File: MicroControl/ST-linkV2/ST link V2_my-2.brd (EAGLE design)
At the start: 57.4 x 22.5 mm, 37 parts, among them IC1 LD117-3.3, Q1 8000 kHz, U1 STM32F103CBT6, X2 CON-PH12-EDGE

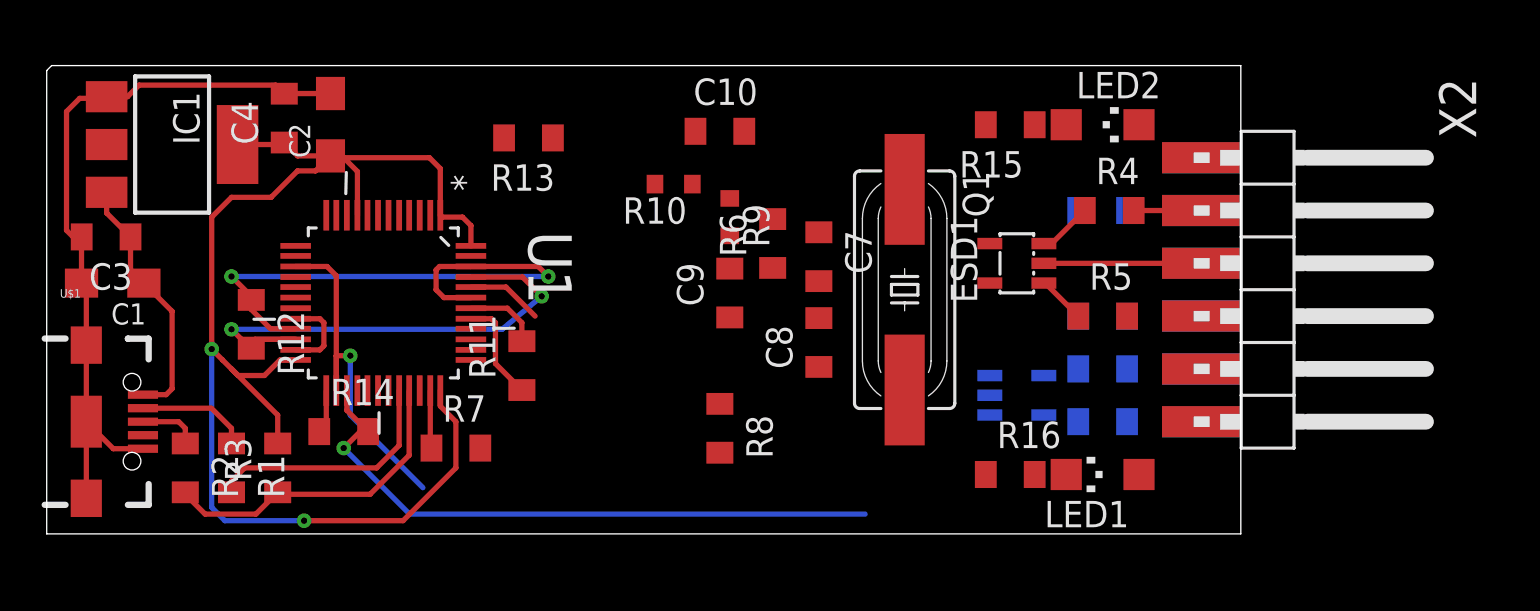
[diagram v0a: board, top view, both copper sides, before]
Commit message: Хорошо
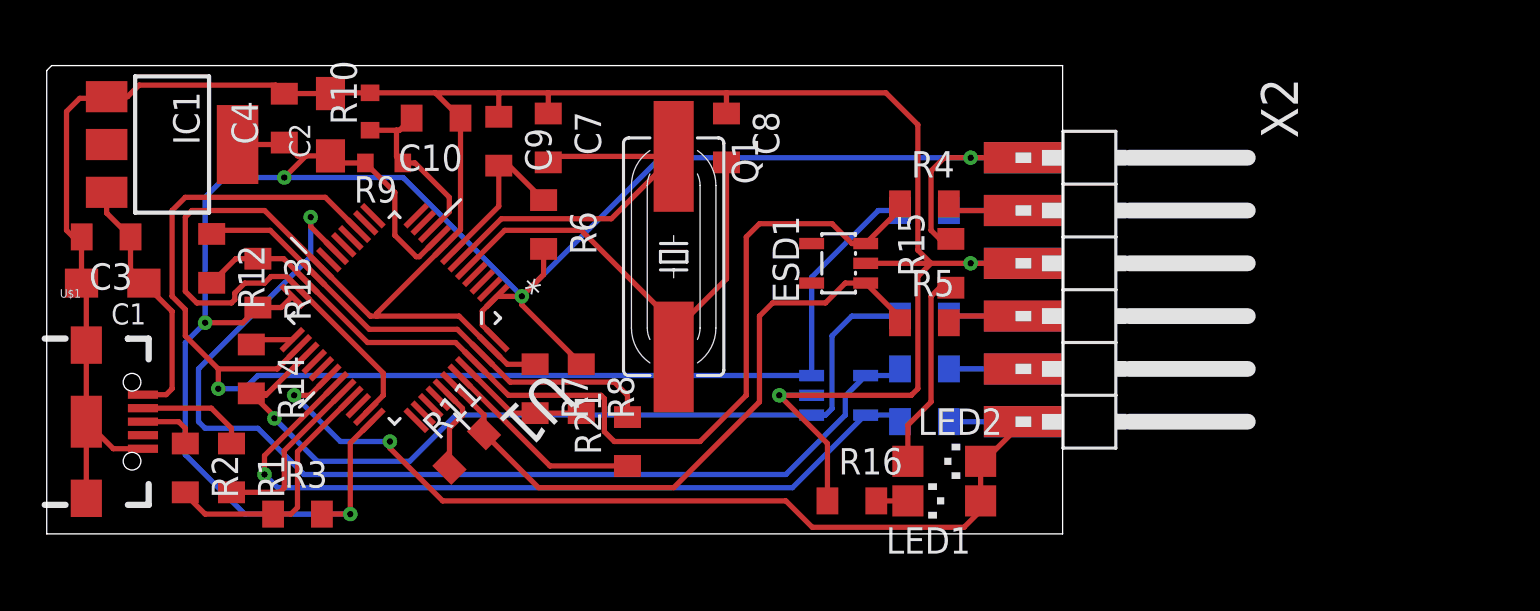
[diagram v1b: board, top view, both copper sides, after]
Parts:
- added R21: 0, Namenlos:R0805
- moved LED2 17.9 mm to (43.2, 3.49)
- moved R9 16.8 mm to (16.2, 17.8), turned to 180 degrees
- moved R10 15.0 mm to (15.6, 20.3), turned to 90 degrees
- moved R13 14.8 mm to (10.2, 12.1), turned to 270 degrees
- moved C7 14.2 mm to (24.1, 19.1)
- moved C10 13.7 mm to (18.7, 20.0), turned to 180 degrees
- moved C9 13.3 mm to (21.7, 18.9), turned to 270 degrees
- moved Q1 11.2 mm to (30.2, 13.3)
- moved R6 11.1 mm to (23.9, 14.9), turned to 270 degrees
- moved C8 10.8 mm to (32.7, 19.1), turned to 270 degrees
- moved R4 8.90 mm to (42.2, 15.9)
- moved R5 8.58 mm to (42.2, 10.2)
- moved ESD1 8.57 mm to (38.1, 13.0)
- moved ESD2 8.57 mm to (38.1, 6.67)
- moved R17 8.57 mm to (42.2, 15.6)
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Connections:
- new net N$17: R21.1, U1.43
- net N$5: now also R21.2; no longer U1.43
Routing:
- net GND: track 50.3 -> 156.9 mm, vias 0 -> 2
- net T_NRST: track 0.00 -> 51.7 mm, vias 0 -> 1
- net +3V3: track 66.9 -> 112.6 mm, vias 2 -> 5
- net T_SWCLK: track 17.8 -> 62.8 mm
- net U1_BL_TX: track 0.00 -> 43.4 mm, vias 0 -> 2
- net U1_BL_RX_T-SWO: track 0.00 -> 38.2 mm, vias 0 -> 1
- net N$6: track 0.00 -> 26.0 mm
- net SWIM_RST: track 5.94 -> 31.6 mm
- net SWIM: track 27.6 -> 48.4 mm, vias 2 -> 0
- net N$7: track 0.00 -> 18.5 mm
- net T_SWDIO: track 30.3 -> 41.2 mm
- net N$17: track 0.00 -> 9.83 mm
- net N$10: track 0.00 -> 9.52 mm
- net N$4: track 0.00 -> 8.82 mm
- net !STMRST: track 0.00 -> 8.25 mm
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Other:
- board size 57.4 x 22.5 mm -> 48.9 x 22.5 mm
